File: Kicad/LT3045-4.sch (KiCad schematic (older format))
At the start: 22 parts, among them J1 Conn_Coaxial_Power, J2 Conn_Coaxial_Power, U1 LT3042, U2 LT3042, U3 LT3042, U4 LT3042

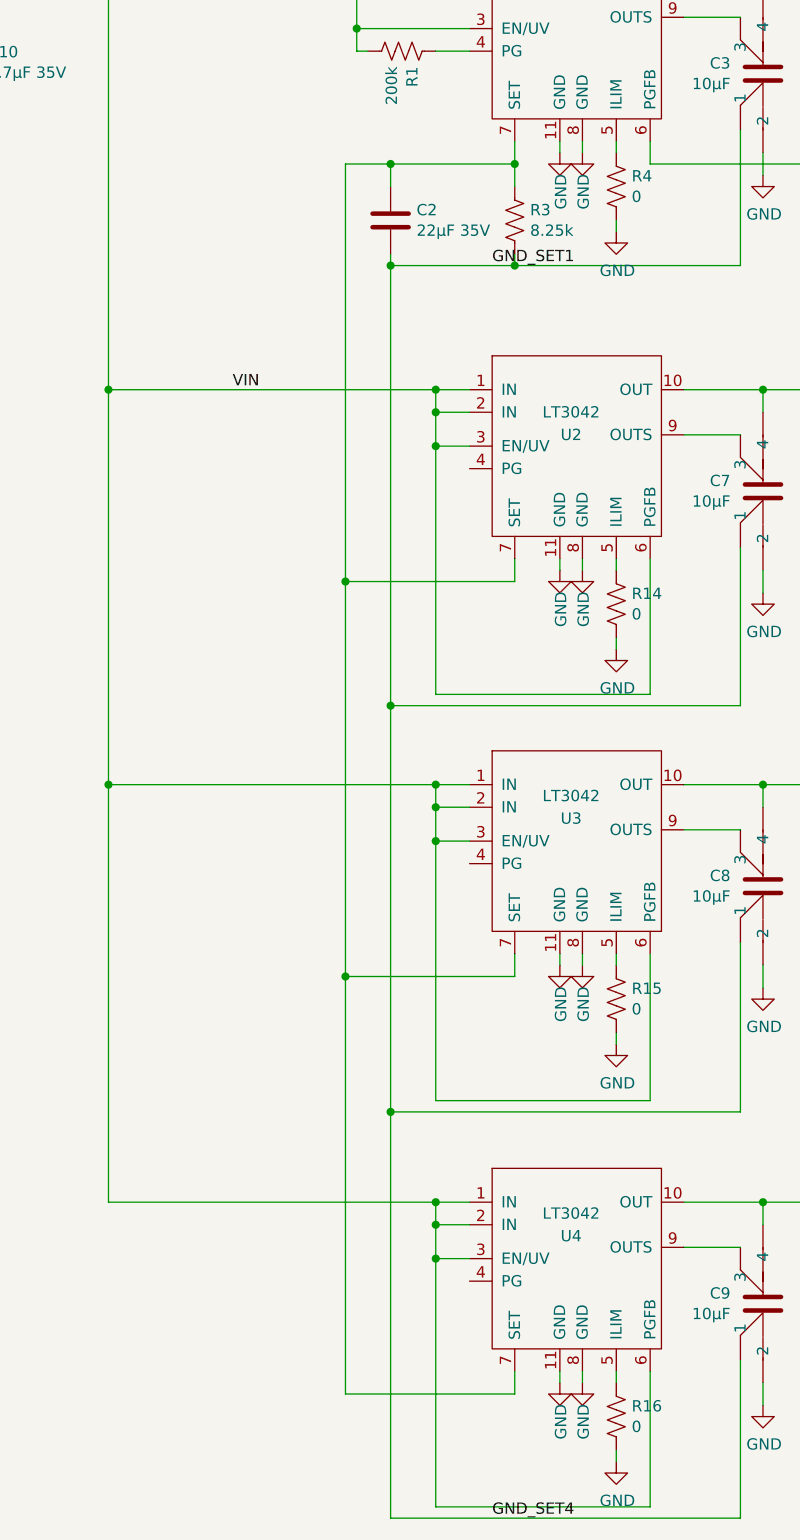
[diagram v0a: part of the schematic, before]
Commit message: VIAS
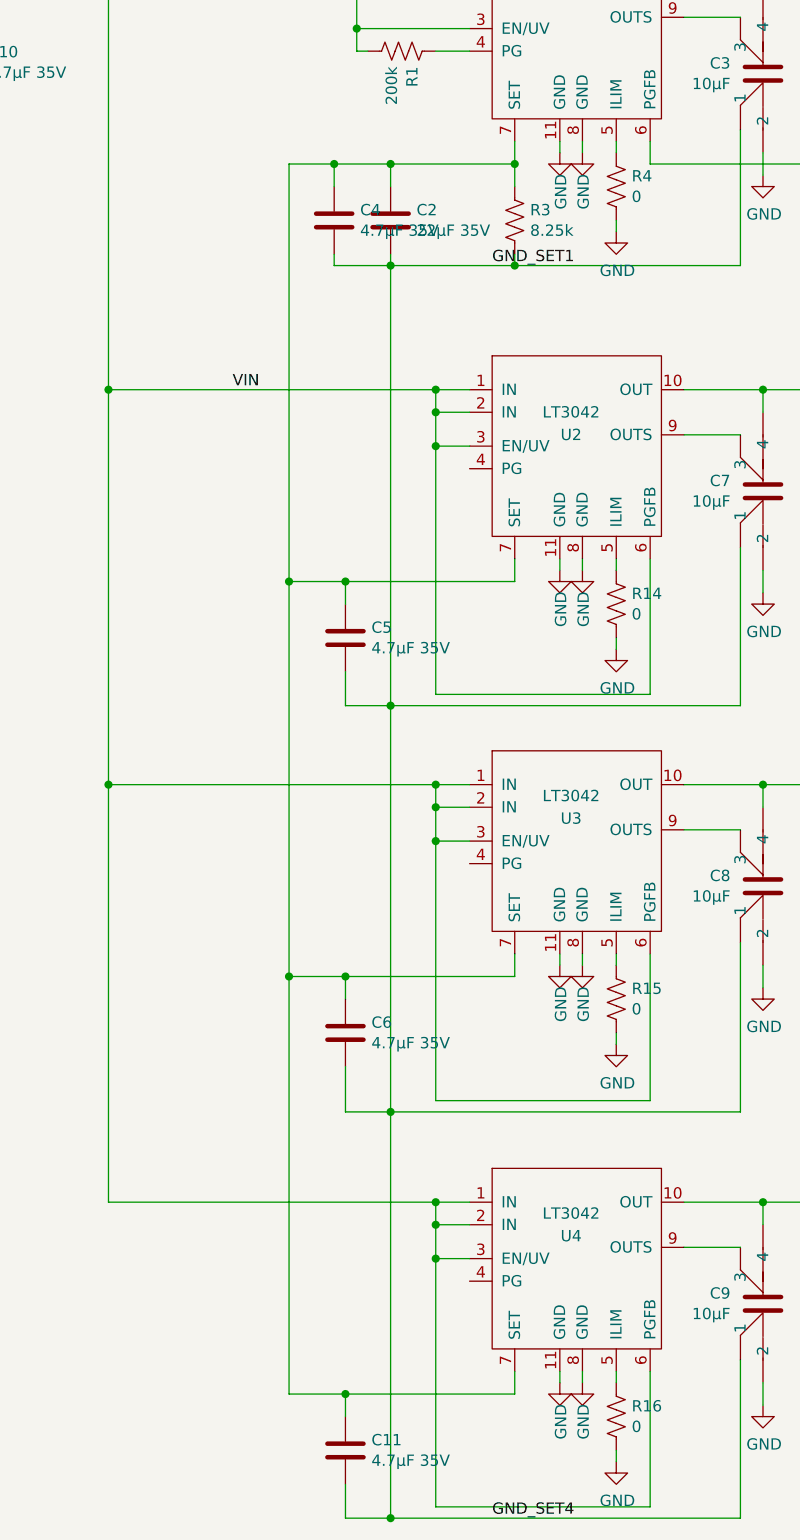
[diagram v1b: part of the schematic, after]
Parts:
- added C11, C4, C5, C6: 4.7µF 35V, Capacitor_SMD:C_0805_2012Metric, symbol Device:C
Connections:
- net GND_SET1: now also C11.2, C4.2, C5.2, C6.2
- net at C2.1, R3.1, U1.7 (SET)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: now also C11.1, C4.1, C5.1, C6.1
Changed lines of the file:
@@
 	2300 1500 1700 1500
-Wire Wire Line
-	4200 1750 4000 1750
-Wire Wire Line
-	4000 1750 4000 3600
 Wire Wire Line
 	4000 3600 4750 3600
@@
 	4750 5250 4750 5350
 Wire Wire Line
-	4750 5350 4000 5350
-Wire Wire Line
-	4000 5350 4000 3600
-Connection ~ 4000 3600
-Wire Wire Line
 	4750 7100 4750 7200
-Wire Wire Line
-	4750 7200 4000 7200
-Wire Wire Line
-	4000 7200 4000 5350
-Connection ~ 4000 5350
 Connection ~ 4200 2200
 Wire Wire Line
@@
 Wire Wire Line
 	5750 3450 5750 4150
+$Comp
+L Device:C C4
+U 1 1 5FD57A1A
+P 3950 2000
+F 0 "C4" H 4065 2046 50  0000 L CNN
+F 1 "4.7µF 35V" H 4065 1955 50  0000 L CNN
+F 2 "Capacitor_SMD:C_0805_2012Metric" H 3988 1850 50  0001 C CNN
+F 3 "~" H 3950 2000 50  0001 C CNN
+	1    3950 2000
+	1    0    0    -1
+$EndComp
+$Comp
+L Device:C C5
+U 1 1 5FD5D837
+P 4000 3850
+F 0 "C5" H 4115 3896 50  0000 L CNN
+F 1 "4.7µF 35V" H 4115 3805 50  0000 L CNN
+F 2 "Capacitor_SMD:C_0805_2012Metric" H 4038 3700 50  0001 C CNN
+F 3 "~" H 4000 3850 50  0001 C CNN
+	1    4000 3850
+	1    0    0    -1
+$EndComp
+$Comp
+L Device:C C6
+U 1 1 5FD6373A
+P 4000 5600
+F 0 "C6" H 4115 5646 50  0000 L CNN
+F 1 "4.7µF 35V" H 4115 5555 50  0000 L CNN
+F 2 "Capacitor_SMD:C_0805_2012Metric" H 4038 5450 50  0001 C CNN
+F 3 "~" H 4000 5600 50  0001 C CNN
+	1    4000 5600
+	1    0    0    -1
+$EndComp
+$Comp
+L Device:C C11
+U 1 1 5FD69ACD
+P 4000 7450
+F 0 "C11" H 4115 7496 50  0000 L CNN
+F 1 "4.7µF 35V" H 4115 7405 50  0000 L CNN
+F 2 "Capacitor_SMD:C_0805_2012Metric" H 4038 7300 50  0001 C CNN
+F 3 "~" H 4000 7450 50  0001 C CNN
+	1    4000 7450
+	1    0    0    -1
+$EndComp
+Wire Wire Line
+	3950 1750 3950 1850
+Connection ~ 3950 1750
+Wire Wire Line
+	3950 1750 4200 1750
+Wire Wire Line
+	4000 3700 4000 3600
+Wire Wire Line
+	3750 1750 3750 3600
+Wire Wire Line
+	3750 3600 4000 3600
+Wire Wire Line
+	3750 1750 3950 1750
+Connection ~ 4000 3600
+Wire Wire Line
+	3750 3600 3750 5350
+Wire Wire Line
+	3750 5350 4000 5350
+Connection ~ 3750 3600
+Wire Wire Line
+	4000 5450 4000 5350
+Connection ~ 4000 5350
+Wire Wire Line
+	4000 5350 4750 5350
+Wire Wire Line
+	4200 5950 4000 5950
+Wire Wire Line
+	4000 5950 4000 5750
+Wire Wire Line
+	4200 4150 4000 4150
+Wire Wire Line
+	4000 4150 4000 4000
+Wire Wire Line
+	4200 2200 3950 2200
+Wire Wire Line
+	3950 2200 3950 2150
+Wire Wire Line
+	3750 5350 3750 7200
+Connection ~ 3750 5350
+Wire Wire Line
+	3750 7200 4000 7200
+Wire Wire Line
+	4000 7300 4000 7200
+Connection ~ 4000 7200
+Wire Wire Line
+	4000 7200 4750 7200
+Wire Wire Line
+	4000 7600 4000 7750
+Wire Wire Line
+	4000 7750 4200 7750
+Connection ~ 4200 7750
 $EndSCHEMATC
